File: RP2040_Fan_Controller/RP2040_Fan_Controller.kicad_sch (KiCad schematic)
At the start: 0 parts

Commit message: PCB-Rev 0.1.0
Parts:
- added A?: RaspberryPi_Pico, Module:RaspberryPi_Pico_Common_Unspecified, symbol MCU_Module:RaspberryPi_Pico
- added Fan1, Fan2, Fan3, Fan4, Fan5, Fan6: Fan_4pin, Connector_PinSocket_2.54mm:PinSocket_1x04_P2.54mm_Horizontal, symbol Motor:Fan_4pin
- added Q10, Q11, Q12, Q7, Q8, Q9: IRLZ44N, Package_TO_SOT_THT:TO-220-3_Vertical, symbol Transistor_FET:IRLZ44N
- added R1, R2, R3: 10k, Resistor_THT:R_Axial_DIN0204_L3.6mm_D1.6mm_P5.08mm_Vertical, symbol Device:R_Small
- added R4, R5, R6, R7, R8, R9: 2.7K, Resistor_THT:R_Axial_DIN0204_L3.6mm_D1.6mm_P5.08mm_Vertical, symbol Device:R_Small
- added TH1, TH2, TH3: 10k, Connector_PinSocket_2.54mm:PinSocket_1x02_P2.54mm_Horizontal, symbol Device:Thermistor_NTC
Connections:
- new net: A?.19 (GPIO14), Q9.1 (G)
- new net: Fan3.1 (-), Q9.3 (S)
- new net: A?.20 (GPIO15), Q10.1 (G)
- new net: Fan4.1 (-), Q10.3 (S)
- new net: Fan4.3 (Tacho), R7.1
- new net: A?.12 (GPIO9), R7.2
- new net: Fan1.1 (-), Q7.3 (S)
- new net: Fan1.3 (Tacho), R4.1
- new net: A?.1 (GPIO0), Fan1.4 (PWM)
- new net: Fan5.1 (-), Q11.3 (S)
- new net: Fan5.3 (Tacho), R8.1
- new net: A?.6 (GPIO4), Fan5.4 (PWM)
- new net: A?.10 (GPIO7), R5.2
- new net: A?.11 (GPIO8), R6.2
- new net: A?.14 (GPIO10), R8.2
- new net: A?.15 (GPIO11), R9.2
- new net: A?.16 (GPIO12), Q7.1 (G)
- new net: A?.17 (GPIO13), Q8.1 (G)
- new net: A?.2 (GPIO1), Fan2.4 (PWM)
- new net: A?.21 (GPIO16), Q12.1 (G)
- new net: A?.22 (GPIO17), Q11.1 (G)
- new net: A?.31 (GPIO26_ADC0), R1.2, TH1.1
- new net: A?.32 (GPIO27_ADC1), R2.2, TH2.1
- new net: A?.33 (AGND), R1.1, R2.1, R3.1
- new net: A?.34 (GPIO28_ADC2), R3.2, TH3.1
- new net: A?.35 (ADC_VREF), TH1.2, TH2.2, TH3.2
- new net: A?.4 (GPIO2), Fan3.4 (PWM)
- new net: A?.5 (GPIO3), Fan4.4 (PWM)
- new net: A?.7 (GPIO5), Fan6.4 (PWM)
- new net: A?.9 (GPIO6), R4.2
- new net: Fan2.1 (-), Q8.3 (S)
- new net: Fan3.3 (Tacho), R6.1
- new net: Fan2.3 (Tacho), R5.1
- new net: Fan6.3 (Tacho), R9.1
- new net: Fan6.1 (-), Q12.3 (S)
- new net +12V: Fan1.2 (+), Fan2.2 (+), Fan3.2 (+), Fan4.2 (+), Fan5.2 (+), Fan6.2 (+)
- new net GND: A?.13 (GND), A?.18 (GND), A?.23 (GND), A?.28 (GND), A?.3 (GND), A?.38 (GND), A?.8 (GND), Q10.2 (D), Q11.2 (D), Q12.2 (D), Q7.2 (D), Q8.2 (D), Q9.2 (D)
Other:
- title: (none) -> RP2040 Fan Controller

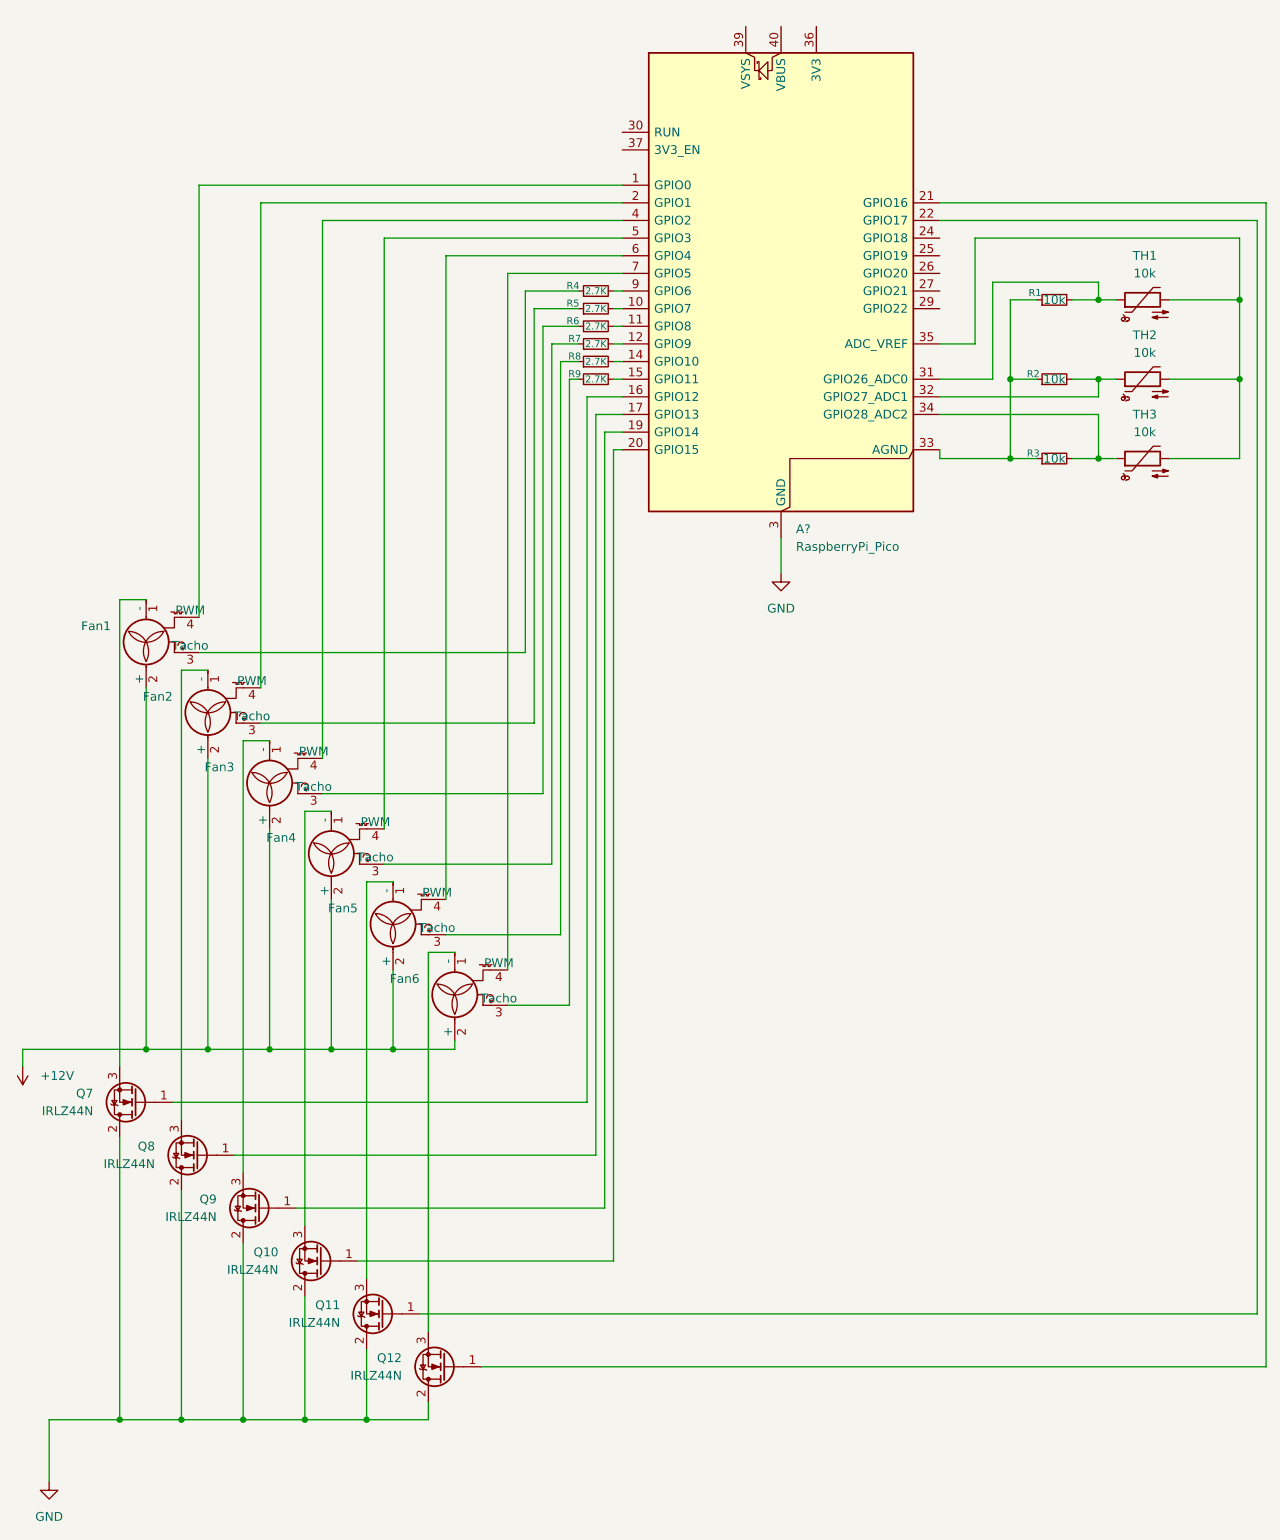
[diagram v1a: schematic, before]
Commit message: PCB-Rev 0.2.0
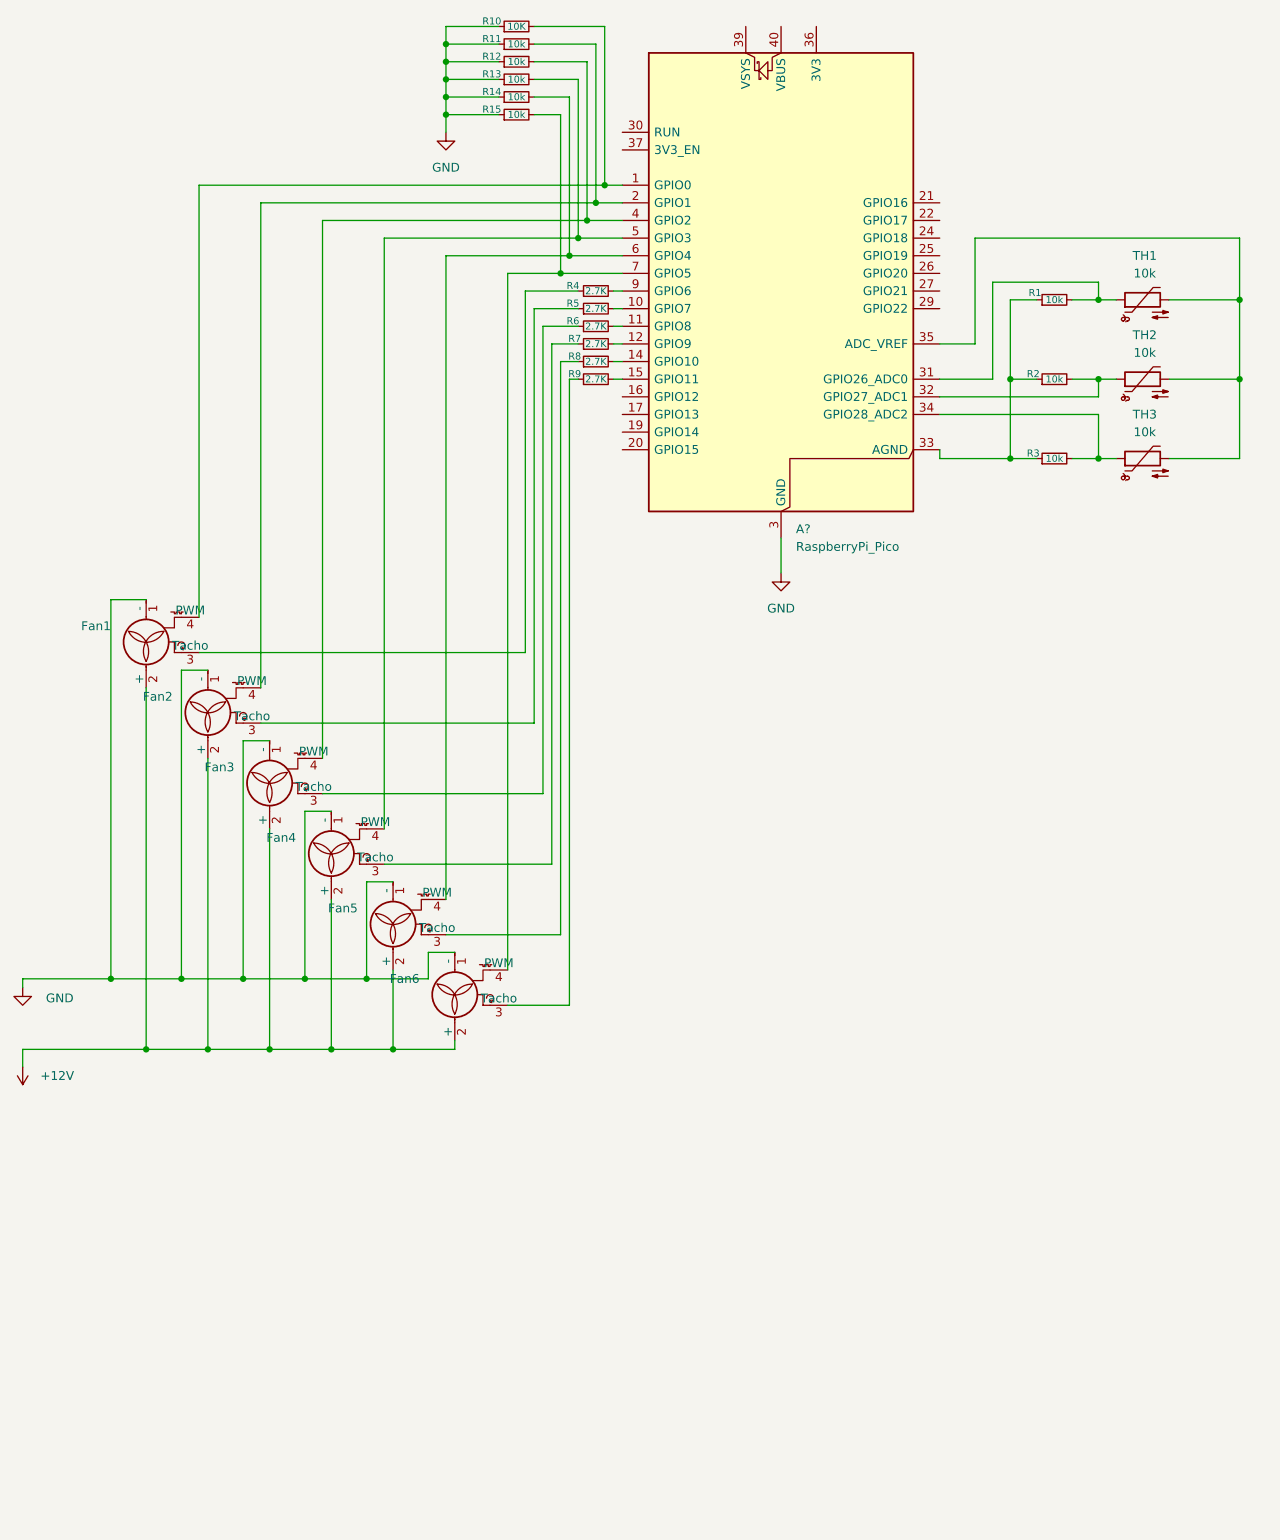
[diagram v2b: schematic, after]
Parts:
- removed Q10, Q11, Q12, Q7, Q8, Q9: IRLZ44N, Package_TO_SOT_THT:TO-220-3_Vertical, symbol Transistor_FET:IRLZ44N
- added R10: 10K, Resistor_THT:R_Axial_DIN0204_L3.6mm_D1.6mm_P5.08mm_Vertical, symbol Device:R_Small
- added R11, R12, R13, R14, R15: 10k, Resistor_THT:R_Axial_DIN0204_L3.6mm_D1.6mm_P5.08mm_Vertical, symbol Device:R_Small
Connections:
- net GND: now also Fan1.1 (-), Fan2.1 (-), Fan3.1 (-), Fan4.1 (-), Fan5.1 (-), Fan6.1 (-), R10.1, R11.1, R12.1, R13.1, R14.1, R15.1
- net at A?.1 (GPIO0), Fan1.4 (PWM): now also R10.2
- net at A?.6 (GPIO4), Fan5.4 (PWM): now also R14.2
- net at A?.2 (GPIO1), Fan2.4 (PWM): now also R11.2
- net at A?.4 (GPIO2), Fan3.4 (PWM): now also R12.2
- net at A?.5 (GPIO3), Fan4.4 (PWM): now also R13.2
- net at A?.7 (GPIO5), Fan6.4 (PWM): now also R15.2
